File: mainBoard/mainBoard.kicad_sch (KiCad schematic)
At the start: 30 parts, among them J1 Battery Output, J2 Conn_01x06_Pin, J3 Keyboard, J4 display, J5 RYLR998, M1 Vibration Motor, Q1 IRLML2502, U1 STM32G030K8Tx, U2 AMS1117-3.3, U3 W25Q128JVS, Y1 48MHz

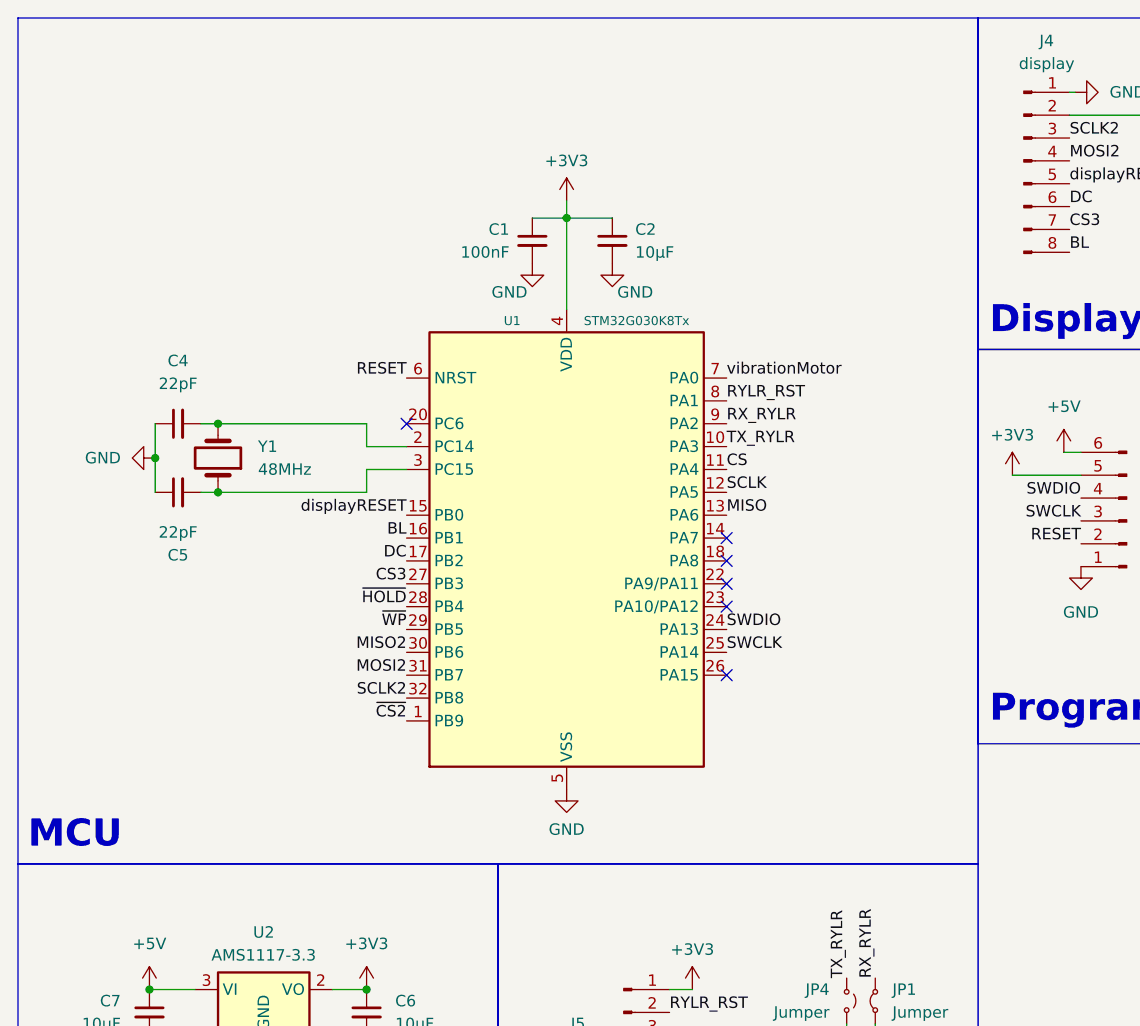
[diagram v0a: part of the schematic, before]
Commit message: Fixed Minor Issue
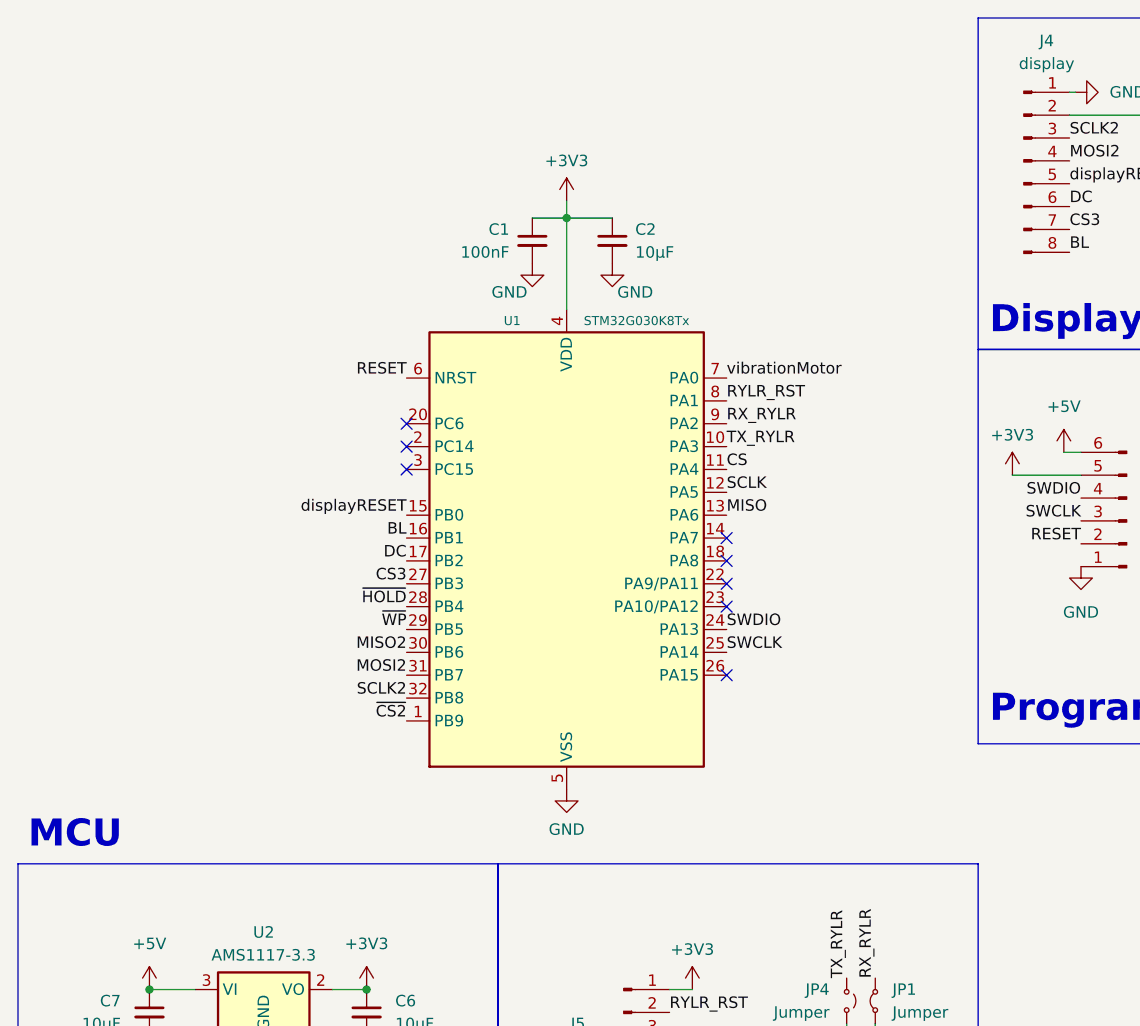
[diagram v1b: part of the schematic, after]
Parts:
- removed C4, C5: 22pF, Capacitor_SMD:C_0603_1608Metric_Pad1.08x0.95mm_HandSolder, symbol Device:C_Small
- removed Y1: 48MHz, Crystal:Crystal_HC49-U_Vertical, symbol Device:Crystal
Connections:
- no-connect marks 6 -> 8
